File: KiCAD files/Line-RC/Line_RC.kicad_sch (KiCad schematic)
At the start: 67 parts, among them IC1 ESP32-WROVER-E-N4R8, IC2 CP2102N-A02-GQFN28R, IC3 BC847BDW1T1G, IC4 TLV75533PDBVR, IC5 TPS563240DDCR, J1 XT60PW-M, J2 XT60PW-M, J3 Conn_01x03_ESC, J4 FFC3B07-08-T, J6 Motor OUT, J7 Motor OUT, U3 DRV8213RTER, U4 DRV8213RTER

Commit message: Validated the repo integrity
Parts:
- removed C13, C17: 47uF/16V, symbol Device:C
- removed C14, C16, C18, C20: 100nF/50V, symbol Device:C
- removed C15, C19: 22nF/50V, symbol Device:C
- removed J6, J7: Motor OUT, symbol Connector_Generic:Conn_01x02
- removed R14, R16: 10k (1%), symbol Device:R
- removed R15, R17: 5k (1%), symbol Device:R
- removed TP6: Vref, symbol Connector:TestPoint
- removed U3, U4: DRV8213RTER, RTE0016C-IPC_A, symbol 2026-07-26_14-19-18:DRV8213RTER
- added C21, C23: 47uF/16V, symbol Device:C
- added C22, C24: 100nF/50V, symbol Device:C
- added J8, J9: Motor OUT, symbol Connector_Generic:Conn_01x02
- added U1, U2: (no value), symbol RZ7899:RZ7899
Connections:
- net +3.3V: now also J4.2; no longer J4.1
- net +BATT: now also C21.1, C22.1, C23.1, C24.1, U1.4 (VCC), U2.4 (VCC)
- net GND: now also J4.1, C21.2, C22.2, C23.2, C24.2, U1.3 (GND), U2.3 (GND); no longer J4.8
- net S0: now also J4.8; no longer J4.3
- net S1: now also J4.7; no longer J4.4
- net S2: now also J4.6; no longer J4.5
- net S3: now also J4.5; no longer J4.6
- net Z: now also J4.4; no longer J4.2
- net ~{E}: now also J4.3; no longer J4.7
- new net: J9.1 (Pin_1), U2.7 (BO), U2.8 (BO)
- new net: J9.2 (Pin_2), U2.5 (FO), U2.6 (FO)
- new net: J8.1 (Pin_1), U1.7 (BO), U1.8 (BO)
- new net: J8.2 (Pin_2), U1.5 (FO), U1.6 (FO)
- new net A1: U2.2 (FI)
- new net A2: U2.1 (BI)
- new net B1: U1.2 (FI)
- new net B2: U1.1 (BI)
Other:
- note added: "Motor driver 2"
- moved on the sheet: C10, C11, C12, C2, C3, C4, C5, C6, C7, C8, C9, IC1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

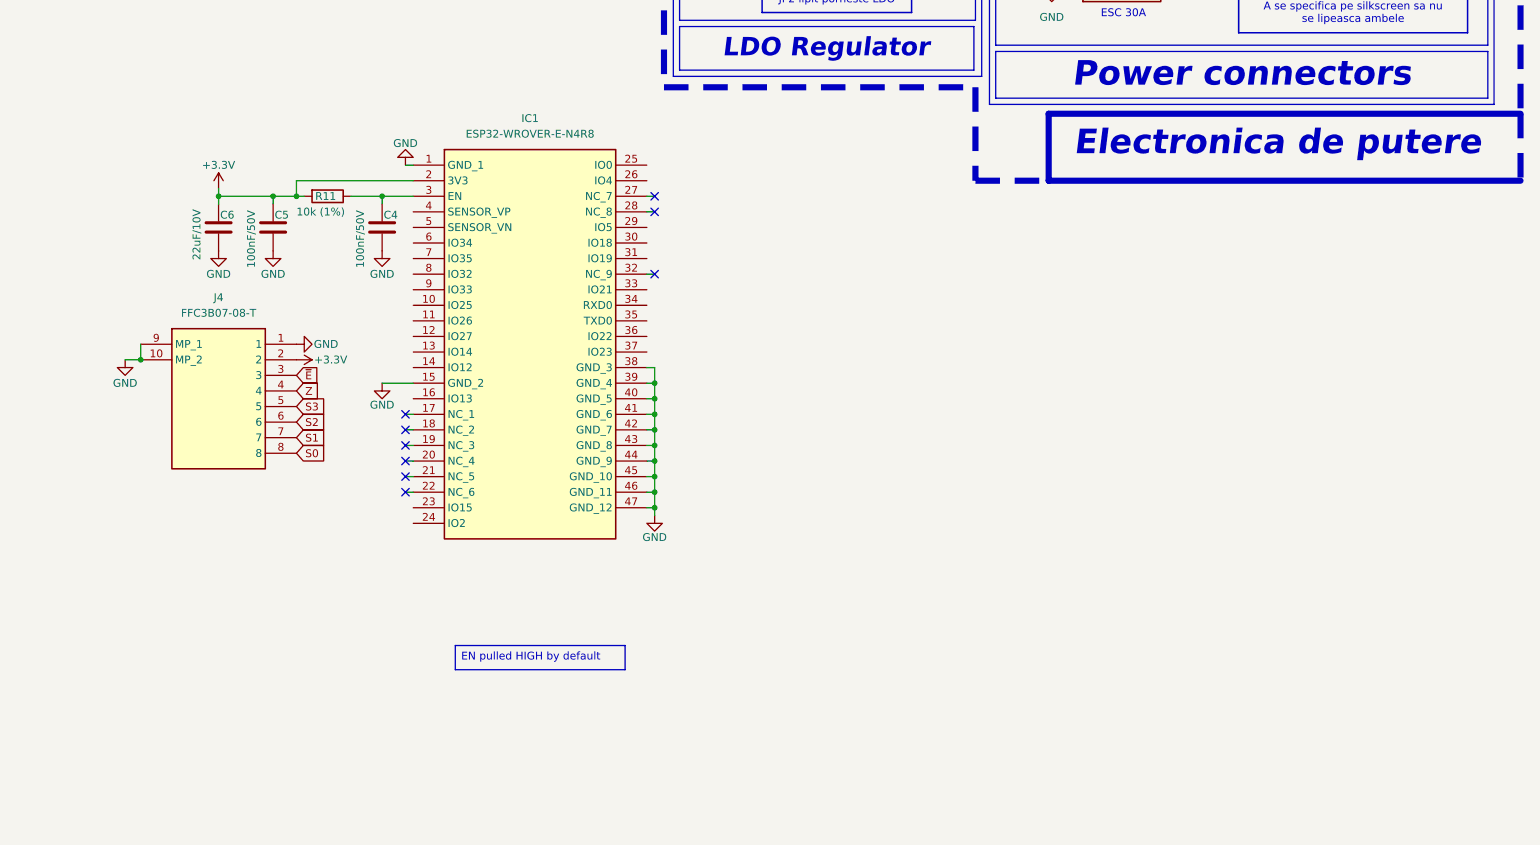
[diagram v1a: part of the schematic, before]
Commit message: Cleanup
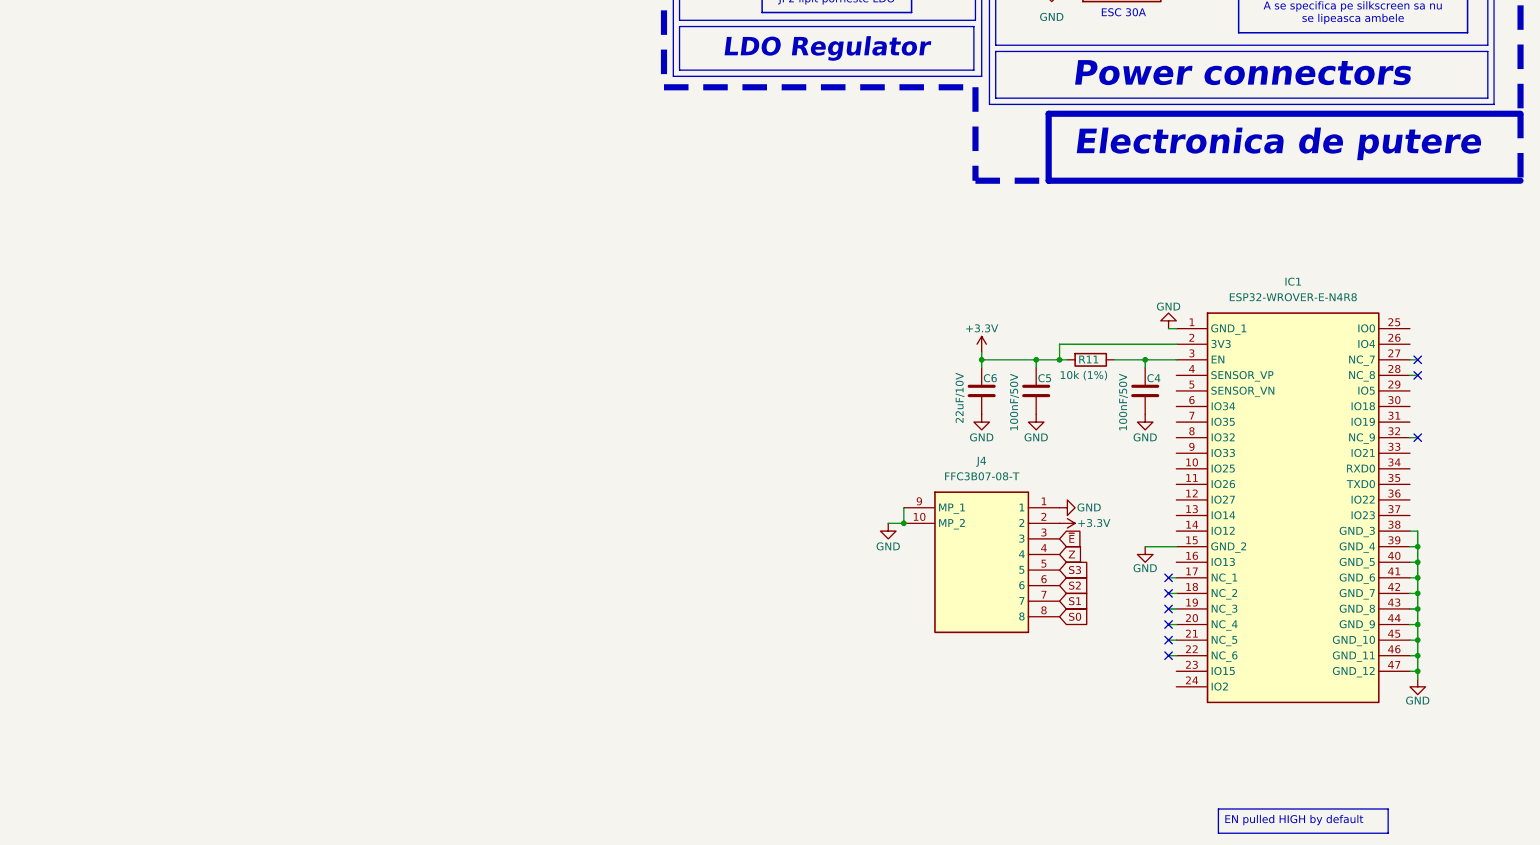
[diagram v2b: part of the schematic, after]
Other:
- moved on the sheet: C4, C5, C6, IC1, J4, R11
